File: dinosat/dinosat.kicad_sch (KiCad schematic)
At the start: 53 parts, among them J1 USB_C_Receptacle_USB2.0_16P, J2 Battery JST, J3 Conn_02x05_Odd_Even, Q1 FS8205A, SW1 SW_Push, SW2 SW_Push, U1 STM32U5A5ZJTx, U2 TP4056-42-ESOP8, U3 DW01A, U4 TPS63060

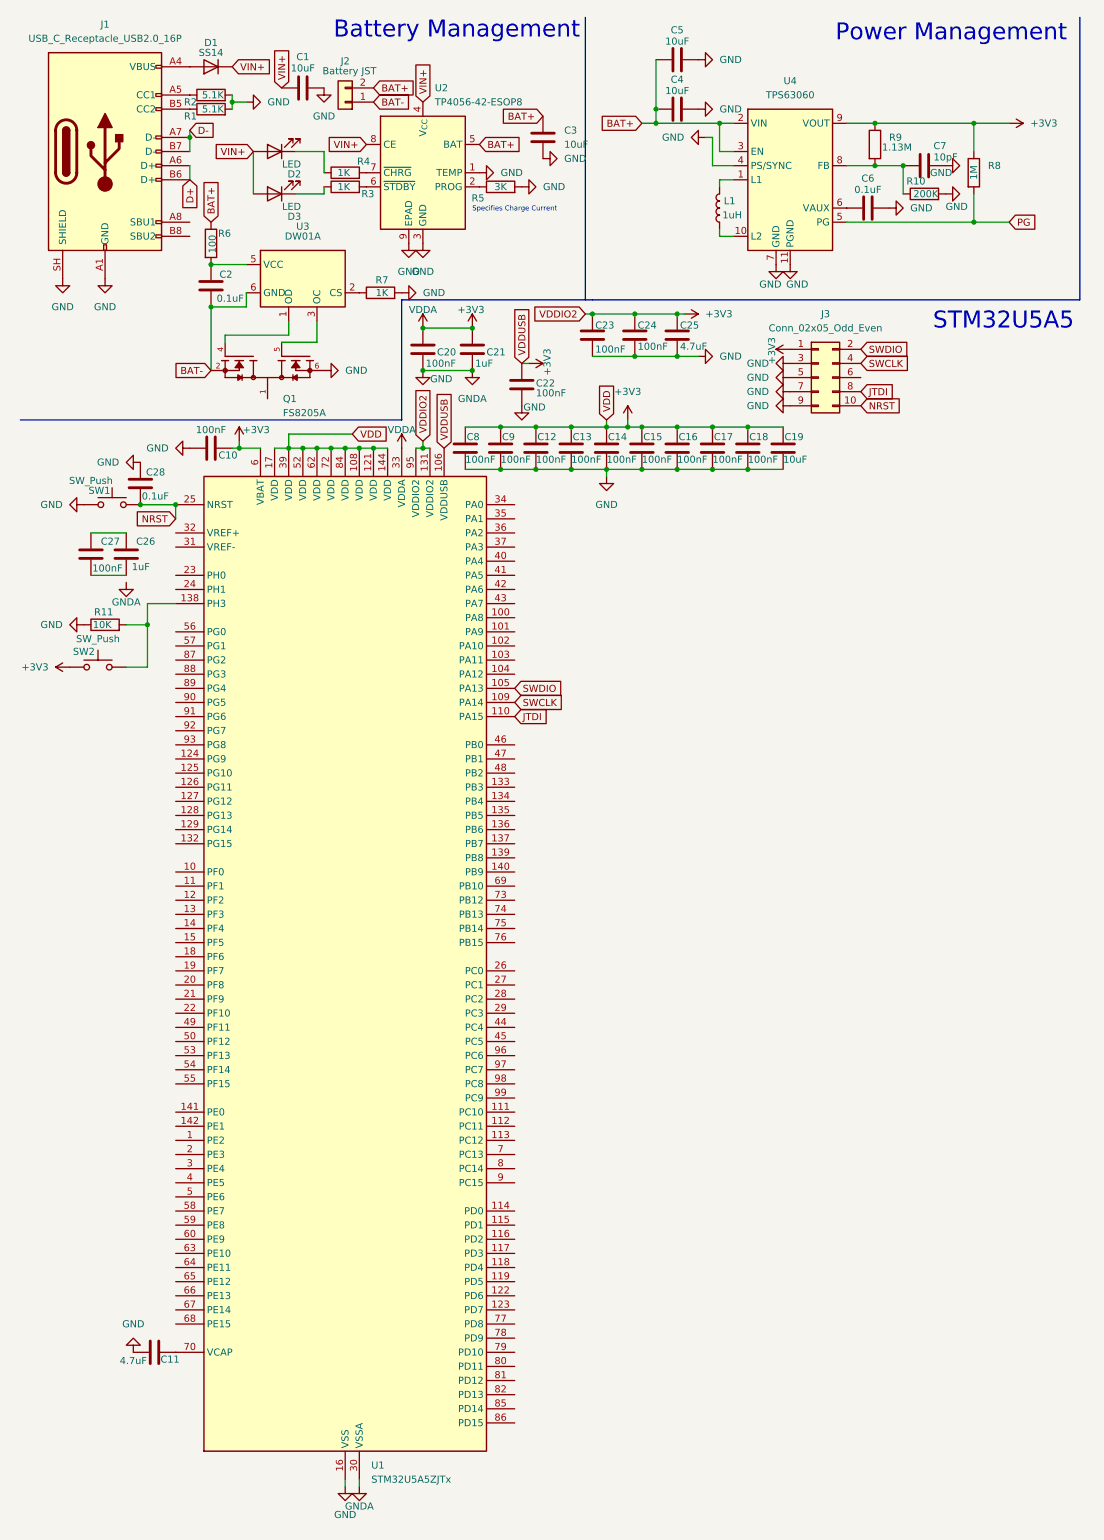
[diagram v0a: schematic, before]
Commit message: Rah
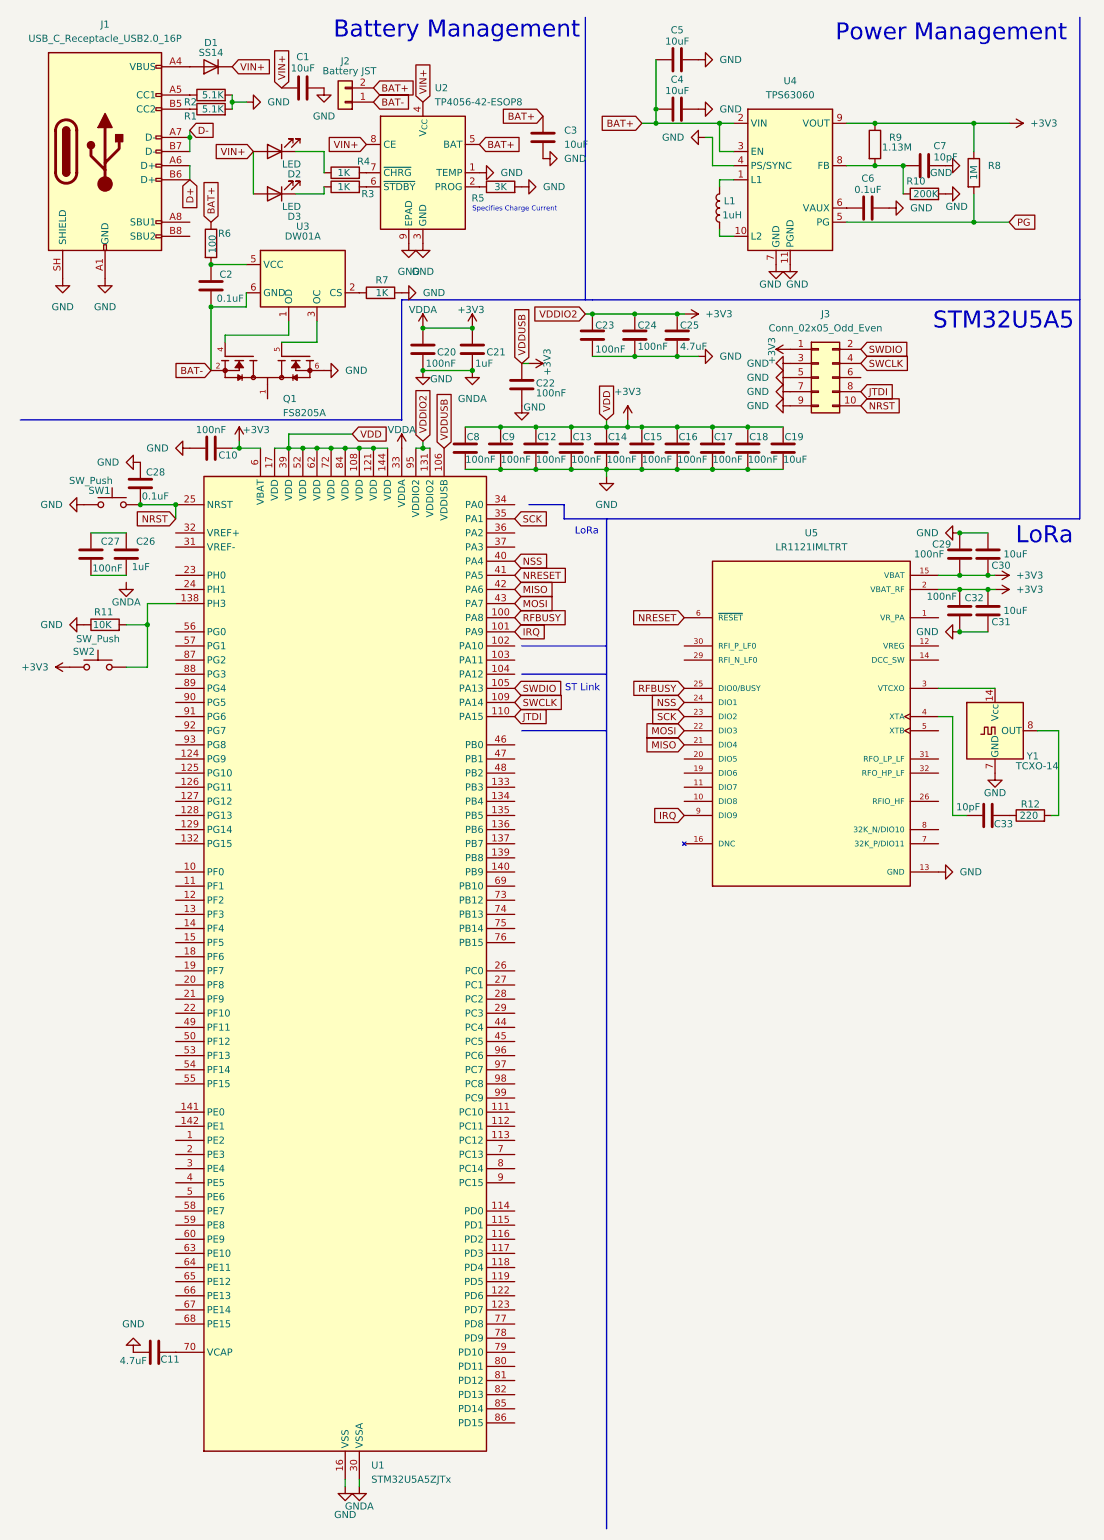
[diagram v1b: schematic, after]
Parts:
- added C29, C32: 100nF, Capacitor_SMD:C_0402_1005Metric, symbol Device:C
- added C30, C31: 10uF, Capacitor_SMD:C_0603_1608Metric, symbol Device:C
- added C33: 10pF, symbol Device:C
- added R12: 220, symbol Device:R
- added U5: LR1121IMLTRT, LR1121IMLTRT:QFN50P500X500X100-33N, symbol LR1121IMLTRT:LR1121IMLTRT
- added Y1: TCXO-14, Oscillator:Oscillator_DIP-14, symbol Oscillator:TCXO-14
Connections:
- net +3V3: now also C29.1, C30.1, C31.2, C32.2, U5.15 (VBAT), U5.2 (VBAT_RF)
- net GND: now also C29.2, C30.2, C31.1, C32.1, U5.13 (GND), U5.33 (GND), Y1.7 (GND)
- net RFBUSY: now reaches U1.100 (PA8)
- net RFBUSY: now also U5.25 (DIO0/BUSY)
- net IRQ: now reaches U1.101 (PA9)
- net IRQ: now also U5.9 (DIO9)
- net SCK: now reaches U1.35 (PA1)
- net SCK: now also U5.23 (DIO2)
- net NSS: now reaches U1.40 (PA4)
- net NSS: now also U5.24 (DIO1)
- net NRESET: now reaches U1.41 (PA5)
- net NRESET: now also U5.6 (~{RESET})
- net MISO: now reaches U1.42 (PA6)
- net MISO: now also U5.21 (DIO4)
- net MOSI: now reaches U1.43 (PA7)
- net MOSI: now also U5.22 (DIO3)
- new net: C33.2, R12.1
- new net: R12.2, Y1.8 (OUT)
- new net: U5.16 (DNC), U5.17 (DNC), U5.18 (DNC), U5.27 (DNC), U5.28 (DNC)
- new net: U5.3 (VTCXO), Y1.14 (Vcc)
- new net: C33.1, U5.4 (XTA)
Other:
- note added: "LoRa"
- note added: "ST Link"
